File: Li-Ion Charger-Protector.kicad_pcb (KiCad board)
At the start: 2 copper layers, 17 parts, among them P1 USB_C_Plug_USB2.0, Q1 FS8205A, U2 TP4056, U3 DW01A

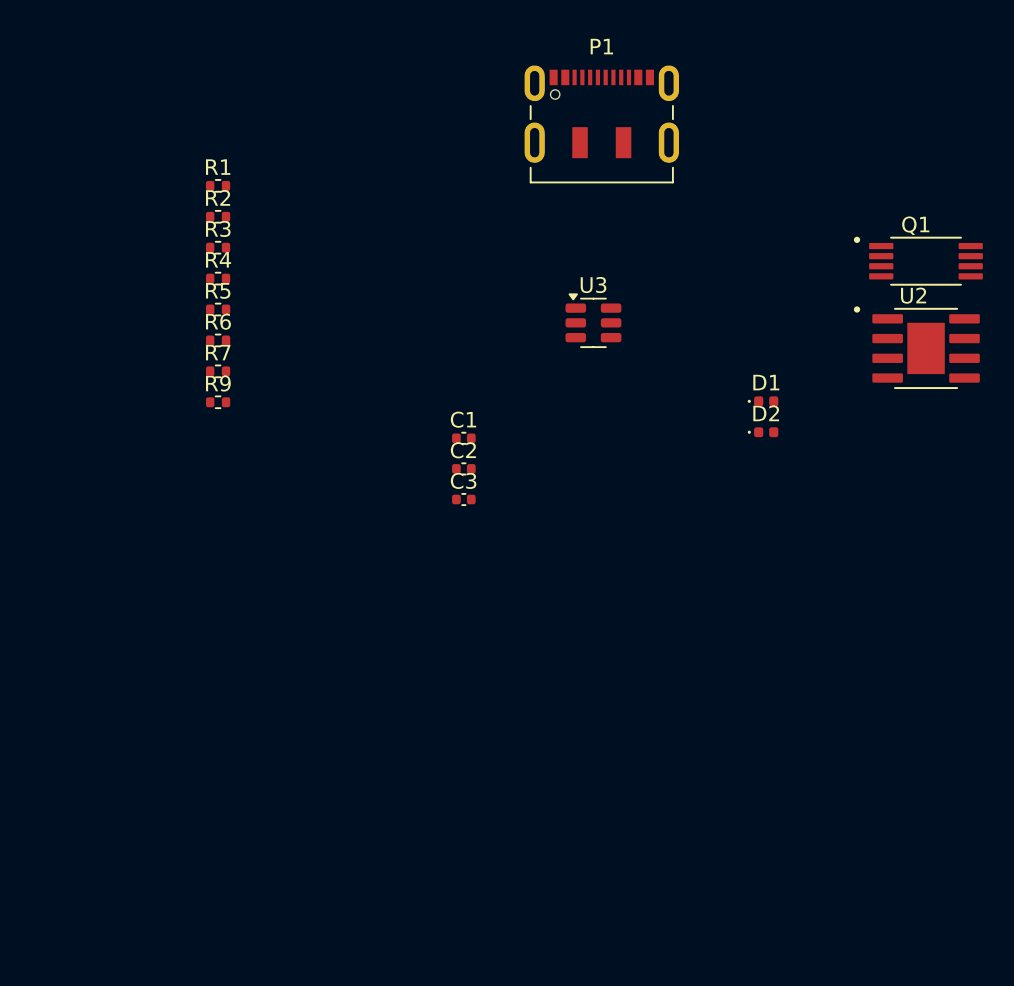
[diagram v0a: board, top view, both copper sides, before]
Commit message: Initial PCB layout; needs work
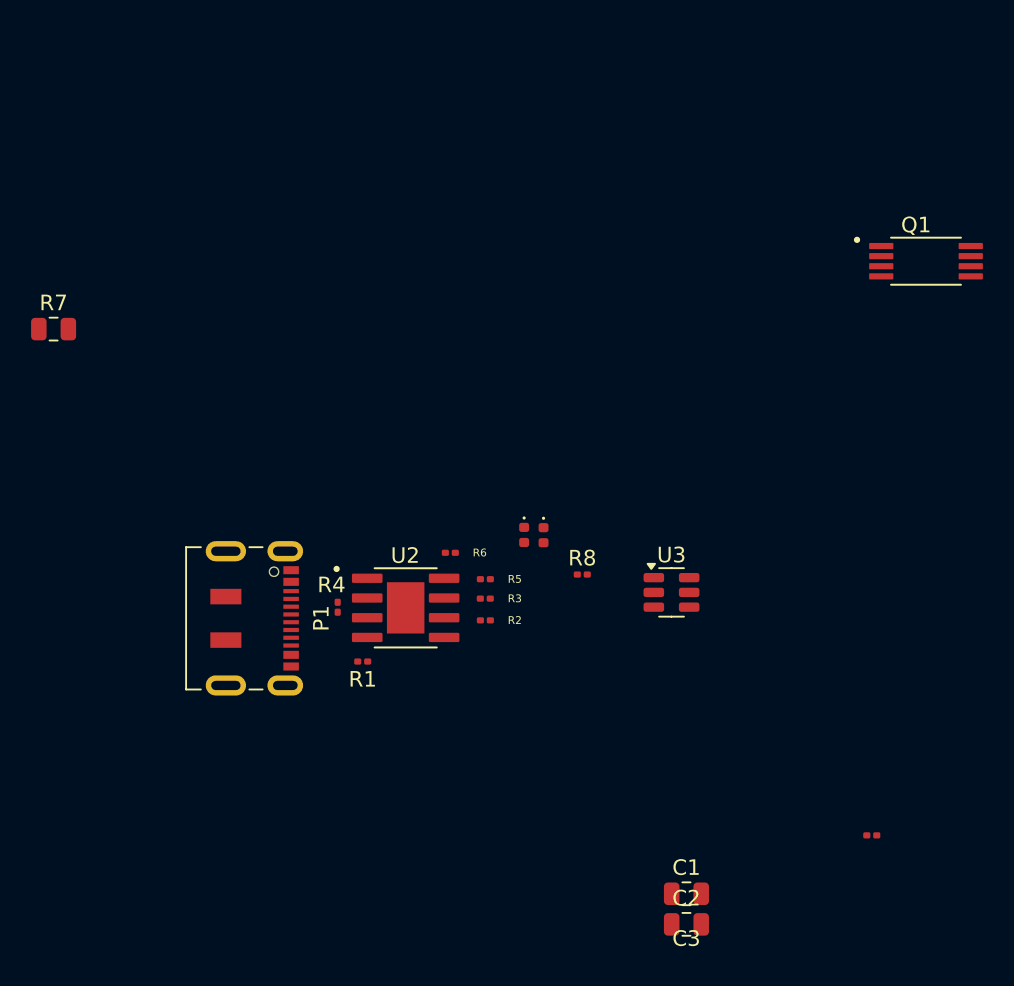
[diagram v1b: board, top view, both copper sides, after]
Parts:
- C1, C2: footprint Capacitor_SMD:C_0402_1005Metric -> Capacitor_SMD:C_0805_2012Metric
- C3: footprint Capacitor_SMD:C_0402_1005Metric -> Capacitor_SMD:C_0201_0603Metric
- R1, R2, R3, R4, R5, R6: footprint Resistor_SMD:R_0402_1005Metric -> Capacitor_SMD:C_0201_0603Metric
- R7: footprint Resistor_SMD:R_0402_1005Metric -> Capacitor_SMD:C_0805_2012Metric
- R8: renamed from R9; footprint Resistor_SMD:R_0402_1005Metric -> Capacitor_SMD:C_0201_0603Metric
- moved P1 39.3 mm to (137.8, 132.4), turned to -90 degrees
- moved U2 37.4 mm to (148.3, 131.7)
- moved C3 34.0 mm to (178.3, 146.3)
- moved C1 32.6 mm to (166.3, 150.1)
- moved C2 32.6 mm to (166.3, 152.1)
- moved R1 32.0 mm to (145.5, 135.2)
- moved R2 31.2 mm to (153.4, 132.5), turned to 180 degrees
- moved R3 28.4 mm to (153.4, 131.1), turned to 180 degrees
- moved R8 25.9 mm to (159.6, 129.6)
- moved R5 24.4 mm to (153.4, 129.8)
- moved R4 22.5 mm to (143.9, 131.7), turned to -90 degrees
- moved R6 20.3 mm to (151.2, 128.2), turned to 180 degrees
- moved U3 18.1 mm to (165.4, 130.7)
- moved D1 17.8 mm to (155.9, 127.0), turned to -90 degrees
- moved D2 15.8 mm to (157.2, 127.0), turned to -90 degrees
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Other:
- copper layers 2 -> 4
